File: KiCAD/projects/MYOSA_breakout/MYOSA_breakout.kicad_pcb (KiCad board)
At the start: 2 copper layers, 259.6 x 142.8 mm, 26 parts, among them J1 Conn_01x04_Socket, J2 Conn_01x05_Socket, J3 PSU_9V, J4 PSU_GND, Q1 IRLZ44N, SW1 Batt/PSU_switch, SW2 USB/REG_switch, U2 D24V22F5

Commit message: MYOSA PCB v1
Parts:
- removed TP4: 3V3_TestPoint, TestPoint:TestPoint_Pad_2.0x2.0mm
- added ?: , , F.Cu at (101.2, 133.6)
- added ?: , , F.Cu at (101.2, 52.6)
- added ?: , , F.Cu at (187.2, 133.3)
- added REF**: MountingHole_2.1mm, MountingHole:MountingHole_2.1mm, F.Cu at (187.2, 52.6)
- BT1, J3, J4: moved to B.Cu
- TP1, TP3, TP5, TP6: footprint TestPoint:TestPoint_Pad_2.0x2.0mm -> TestPoint:TestPoint_Loop_D2.50mm_Drill1.85mm
- moved U2 129.3 mm to (176.5, 108.5), turned to -90 degrees
- moved R_reg_LED1 124.4 mm to (165.9, 116.8), turned to -90 degrees
- moved R_ADC_pulldown1 118.8 mm to (159.9, 101.6), turned to 90 degrees
- moved C_Vin1 112.5 mm to (155.3, 125.4), turned to 180 degrees
- moved R_Vin1 107.0 mm to (146.0, 125.5), turned to 180 degrees
- moved C_ADC_cap1 104.7 mm to (155.7, 101.5), turned to 90 degrees
- moved 5V_Reg_LED1 101.4 mm to (182.8, 116.7), turned to 180 degrees
- moved BT1 92.4 mm to (140.5, 120.6), turned to 90 degrees
- moved TP6 79.7 mm to (124.5, 126.6)
- moved Q1 79.1 mm to (105.3, 115.5), turned to 90 degrees
- moved TP3 78.8 mm to (118.8, 126.8)
- moved R_FET_pulldown1 78.6 mm to (115.0, 116.7), turned to 90 degrees
- moved SW_BAT/PSU1 74.2 mm to (149.3, 113.3), turned to 180 degrees
- moved R_FET_Gate1 72.8 mm to (110.4, 109.0), turned to -90 degrees
- moved R_series_MWIR_LED1 72.0 mm to (117.4, 81.8), turned to 90 degrees
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- renumbered D1 to 5V_Reg_LED1, J1 to CON_BMP180_1, J2 to CON_LED_Photodiode1, C2 to C_3V3_out1, ADC_cap1 to C_ADC_cap1, C1 to C_Vin1, ADC_pulldown1 to R_ADC_pulldown1, R2 to R_FET_Gate1, R3 to R_FET_pulldown1, R5 to R_Vin1, R4 to R_reg_LED1, R1 to R_series_MWIR_LED1, SW1 to SW_BAT/PSU1, SW2 to SW_USB1
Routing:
- net /5V: track 0.00 -> 115.8 mm, vias 0 -> 2
- net /Photo_IN: track 0.00 -> 107.1 mm, vias 0 -> 2
- net /LED_Anode: track 0.00 -> 58.4 mm, vias 0 -> 1
- net /CLK: track 0.00 -> 53.5 mm, vias 0 -> 2
- net /PWM: track 0.00 -> 53.5 mm
- net /3V3_OUT: track 0.00 -> 49.8 mm
- net /DAT: track 0.00 -> 46.5 mm, vias 0 -> 2
- net Net-(J3-Pin_1): track 0.00 -> 46.1 mm
- net /LED_Cathode: track 0.00 -> 43.5 mm
- net /Vin_SRC: track 0.00 -> 26.5 mm
- net Net-(Q1-G): track 0.00 -> 21.3 mm
- net Net-(5V_Reg_LED1-A): track 0.00 -> 20.4 mm
- net Net-(SW_USB1-C): track 0.00 -> 14.8 mm
- net Net-(BT1-+): track 0.00 -> 9.36 mm
- net Net-(C_Vin1-Pad2): track 0.00 -> 4.27 mm
- added copper zone on B.Cu, net GND
- added copper zone on F.Cu, net GND
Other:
- board size 259.6 x 142.8 mm -> 94.3 x 87.4 mm
- board text added: "+-"
- board text added: "100"
- board text added: "100k"
- board text added: "100n"
- board text added: "1k"
- board text added: "200"
- board text added: "3R4"
- board text added: "3V3"
- board text added: "5V"
- board text added: "CLK"
- board text added: "DAT"
- board text added: "DAT x x CLK x"
- board text added: "GND"
- board text added: "LED+"
- board text added: "LED-"
- board text added: "MYOSA USB|VIN"
- board text added: "PERIPH. BAT|PSU"
- board text added: "PWM"
- board text added: "Photo"
- board text added: "v"

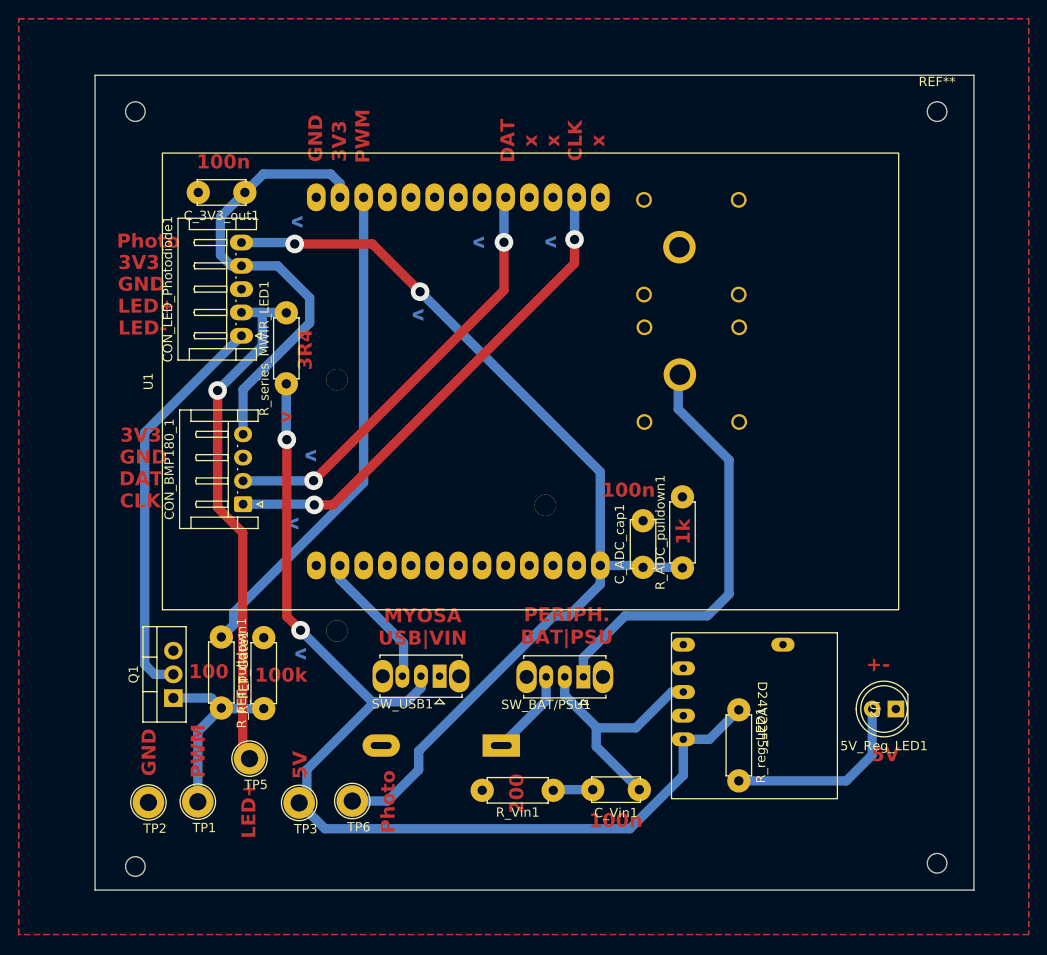
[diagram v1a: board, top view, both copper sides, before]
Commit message: KiCAD Updates + Manufacturing
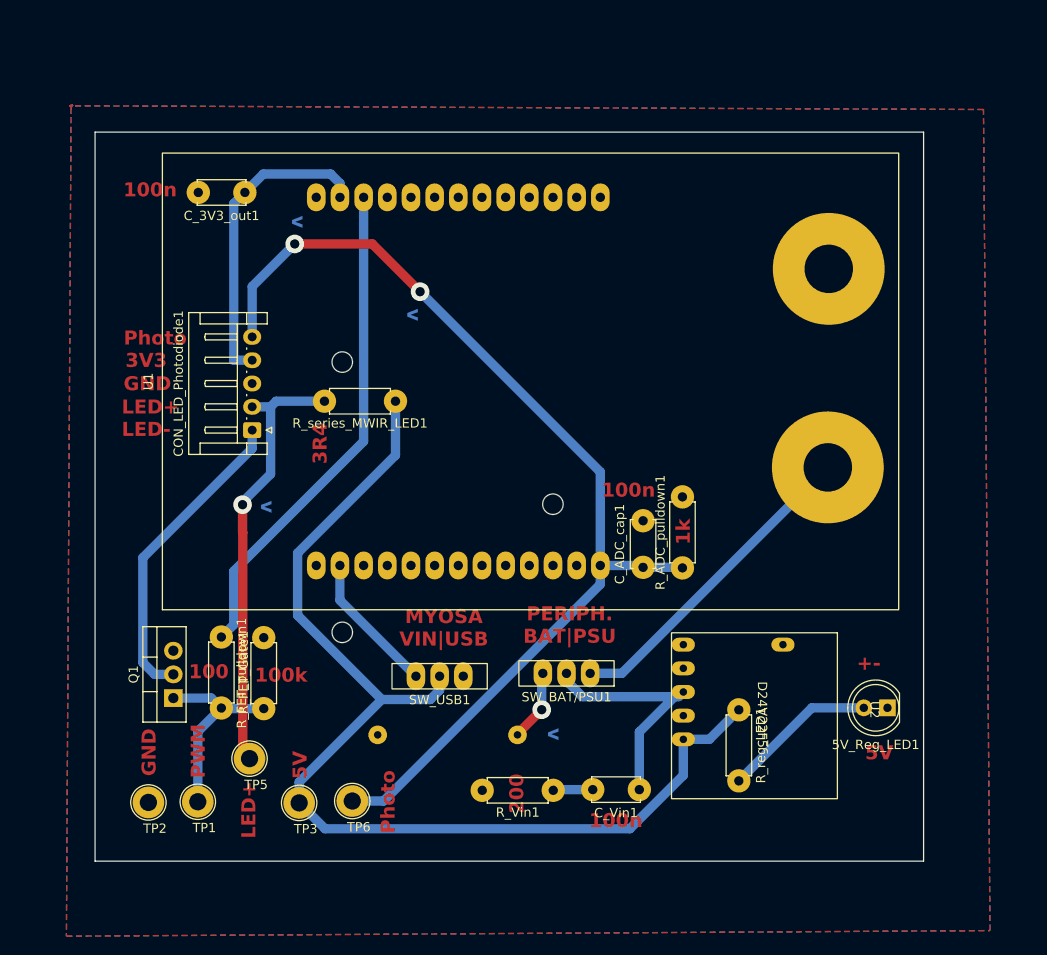
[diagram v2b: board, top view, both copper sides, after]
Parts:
- removed ? (x3): , 
- removed CON_BMP180_1: Conn_01x04_Socket, Connector_JST:JST_EH_S4B-EH_1x04_P2.50mm_Horizontal
- removed REF**: MountingHole_2.1mm, MountingHole:MountingHole_2.1mm
- J3: footprint Connector:Banana_Cliff_FCR7350R_S16N-PC_Horizontal -> Connector:Banana_Jack_1Pin
- J4: footprint Connector:Banana_Cliff_FCR7350B_S16N-PC_Horizontal -> Connector:Banana_Jack_1Pin
- SW_BAT/PSU1, SW_USB1: footprint Button_Switch_THT:SW_Slide_SPDT_Straight_CK_OS102011MS2Q -> Button_Switch_THT:SW_Slide-03_Wuerth-WS-SLTV_10x2.5x6.4_P2.54mm
- moved BT1 20.8 mm to (119.7, 122.5), turned to 0 degrees
- moved J3 18.7 mm to (175.5, 90.8)
- moved J4 16.2 mm to (175.6, 69.5)
- moved R_series_MWIR_LED1 11.9 mm to (129.1, 83.7), turned to 180 degrees
- moved CON_LED_Photodiode1 10.2 mm to (113.7, 86.8)
- moved SW_BAT/PSU1 1.85 mm to (147.5, 112.9)
- moved 5V_Reg_LED1 0.91 mm to (181.9, 116.6)
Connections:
- U1 pad 15: /CLK -> unconnected-(U1-SCL-Pad15)
- U1 pad 18: /DAT -> unconnected-(U1-SDA-Pad18)
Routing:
- net /CLK: track 53.5 -> 0.00 mm, vias 2 -> 0
- net /DAT: track 46.5 -> 0.00 mm, vias 2 -> 0
- net /3V3_OUT: track 49.8 -> 33.4 mm
- net Net-(J3-Pin_1): track 46.1 -> 34.7 mm
- net /LED_Anode: track 58.4 -> 47.3 mm
- net /LED_Cathode: track 43.5 -> 34.1 mm
- net /Photo_IN: track 107.1 -> 112.2 mm
- net Net-(5V_Reg_LED1-A): track 20.4 -> 16.7 mm
- net /5V: track 115.8 -> 118.9 mm, vias 2 -> 0
- net Net-(BT1-+): track 9.36 -> 7.73 mm, vias 0 -> 1
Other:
- board size 94.3 x 87.4 mm -> 88.9 x 78.2 mm
- board text added: "MYOSA VIN|USB"
- board text removed: "CLK"
- board text removed: "DAT"
- board text removed: "DAT x x CLK x"
- board text removed: "MYOSA USB|VIN"
